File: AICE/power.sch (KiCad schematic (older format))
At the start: 58 parts, among them J8 USB_B_Micro, U13 ZLDO1117G33TA, U14 ZLDO1117G12TA, U15 ZLDO1117G33TA, U16 ZLDO1117G18TA, U17 XC6206P282MR, U18 XC6206P152MR

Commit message: Add files via upload
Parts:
- C34, C35, C40, C41, C45, C46, C49, C50, C53, C54, C57, C58: footprint Capacitor_SMD:C_0805_2012Metric_Pad1.15x1.40mm_HandSolder -> Capacitor_SMD:C_0805_2012Metric
- C36, C37, C39, C42, C43, C44, C47, C48, C51, C52, C55, C56, C59, C60: footprint Capacitor_SMD:C_0603_1608Metric_Pad1.05x0.95mm_HandSolder -> Capacitor_SMD:C_0603_1608Metric
- C38: footprint Capacitor_SMD:C_1206_3216Metric_Pad1.42x1.75mm_HandSolder -> Capacitor_SMD:C_1206_3216Metric
- D10, D11, D12, D13, D7, D8, D9: footprint LED_SMD:LED_0603_1608Metric_Pad1.05x0.95mm_HandSolder -> LED_SMD:LED_0603_1608Metric
- L2, L3, L4, L5, L6, L7: footprint Inductor_SMD:L_0805_2012Metric_Pad1.15x1.40mm_HandSolder -> Inductor_SMD:L_0805_2012Metric
- R100, R101, R95, R96, R97, R98, R99: footprint Resistor_SMD:R_0603_1608Metric_Pad1.05x0.95mm_HandSolder -> Resistor_SMD:R_0603_1608Metric

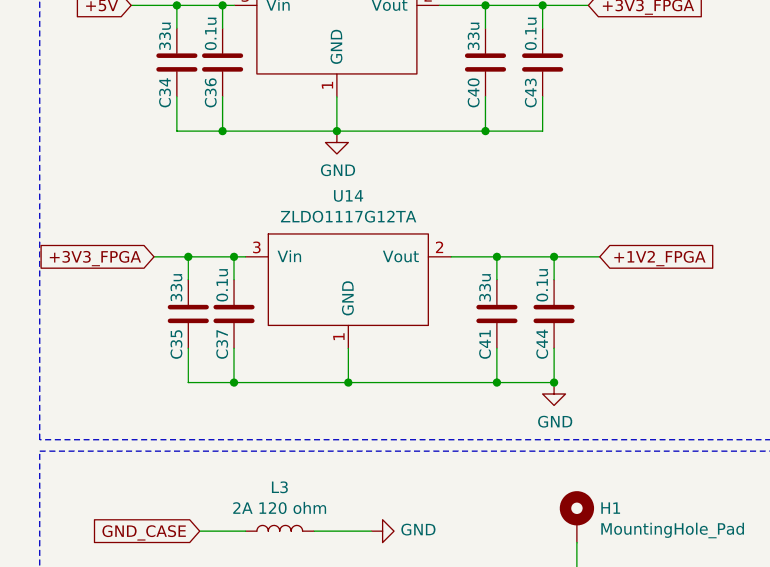
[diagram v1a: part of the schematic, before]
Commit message: Add files via upload
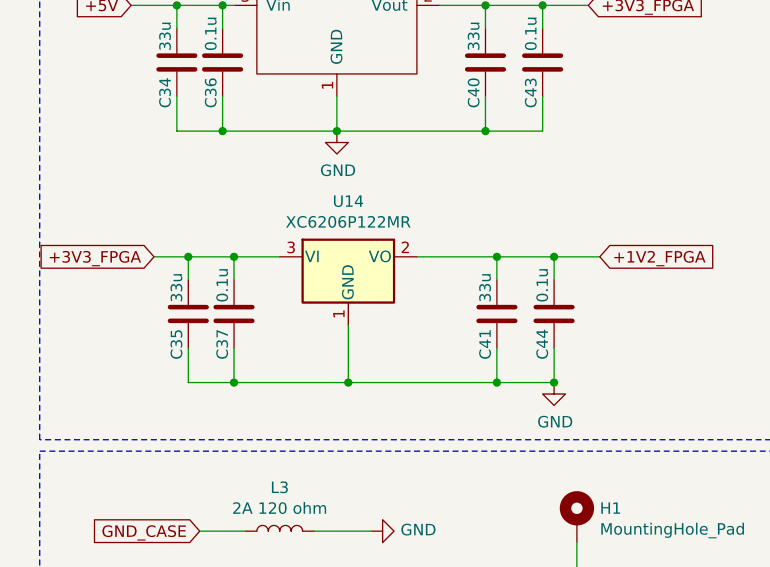
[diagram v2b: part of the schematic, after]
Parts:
- removed U14: ZLDO1117G12TA, Package_TO_SOT_SMD:SOT-223, symbol LDO:ZLDO1117G12TA
- added U14: XC6206P122MR, Package_TO_SOT_SMD:SOT-23, symbol Regulator_Linear:XC6206PxxxMR
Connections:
- net +1V2_FPGA: now also U14.2 (VO)
- net +3V3_FPGA: now also U14.3 (VI)
- net GND: now also U14.1 (GND)
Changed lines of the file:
@@
 $EndComp
-Wire Wire Line
-	1700 3950 1650 3950
 Wire Wire Line
 	1450 4050 1450 3950
@@
 Wire Wire Line
 	2800 4500 3050 4500
-Wire Wire Line
-	2150 4350 2150 4500
 Connection ~ 2150 4500
 Wire Wire Line
 	2150 4500 2800 4500
-Wire Wire Line
-	2600 3950 2800 3950
 Wire Wire Line
 	3050 4050 3050 3950
@@
 	1    0    0    -1
 $EndComp
-$Comp
-L LDO:ZLDO1117G12TA U14
-U 1 1 5EA7B8AA
-P 2150 4050
-F 0 "U14" H 2150 4415 50  0000 C CNN
-F 1 "ZLDO1117G12TA" H 2150 4324 50  0000 C CNN
-F 2 "Package_TO_SOT_SMD:SOT-223" H 2200 4500 50  0001 C CNN
-F 3 "" H 2150 4050 50  0001 C CNN
-	1    2150 4050
-	1    0    0    -1
-$EndComp
 Wire Wire Line
 	1350 1700 1350 1900
@@
 Wire Wire Line
 	3400 1100 3600 1100
+$Comp
+L Regulator_Linear:XC6206PxxxMR U14
+U 1 1 5EC5F7A3
+P 2150 3950
+F 0 "U14" H 2150 4192 50  0000 C CNN
+F 1 "XC6206P122MR" H 2150 4101 50  0000 C CNN
+F 2 "Package_TO_SOT_SMD:SOT-23" H 2150 4175 50  0001 C CIN
+F 3 "https://www.torexsemi.com/file/xc6206/XC6206.pdf" H 2150 3950 50  0001 C CNN
+	1    2150 3950
+	1    0    0    -1
+$EndComp
+Wire Wire Line
+	2450 3950 2800 3950
+Wire Wire Line
+	2150 4250 2150 4500
+Wire Wire Line
+	1650 3950 1850 3950
 $EndSCHEMATC
